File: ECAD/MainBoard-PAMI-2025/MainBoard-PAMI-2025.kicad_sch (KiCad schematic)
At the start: 52 parts, among them J10 Serial, J11 Con_Batt, J13 OLED, J2 USB_B, J3 Sensor_RIGHT, J4 Servo, J5 Sensor_LEFT, J6 Servo, J7 LeftMotor, J8 RightMotor, SW1 SW_SPDT, SW2 SW_Reed, SW3 SW_SPDT, SW4 SW_DIP_x02, U1 ESP32-S3-WROOM-1, U3 TMC2208_SILENTSTEPSTICK, U4 TMC2208_SILENTSTEPSTICK, U5 R-78E3.3-1.0

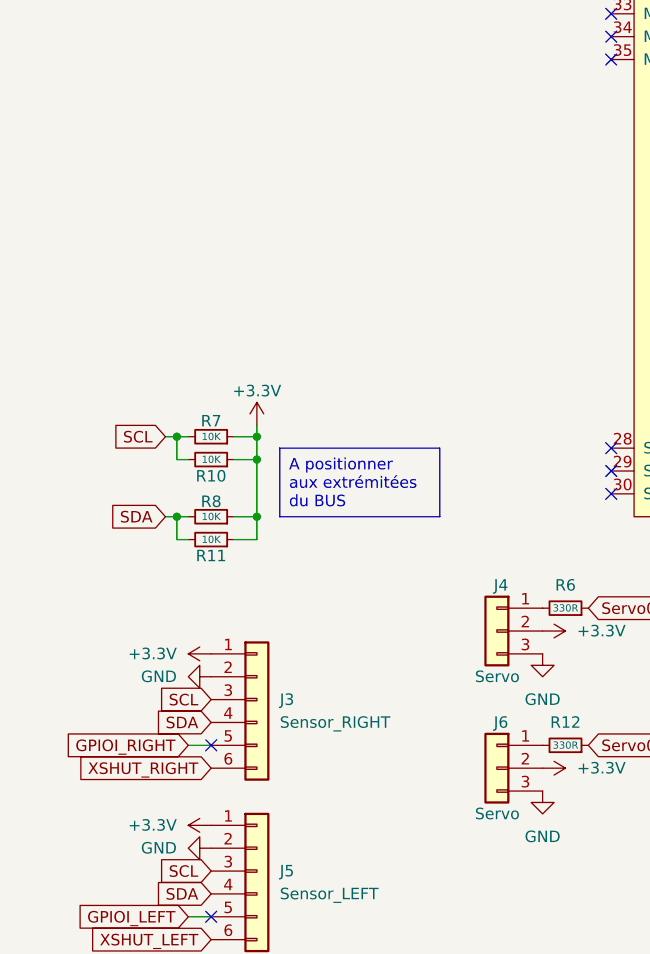
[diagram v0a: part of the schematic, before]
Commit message: add sensor center
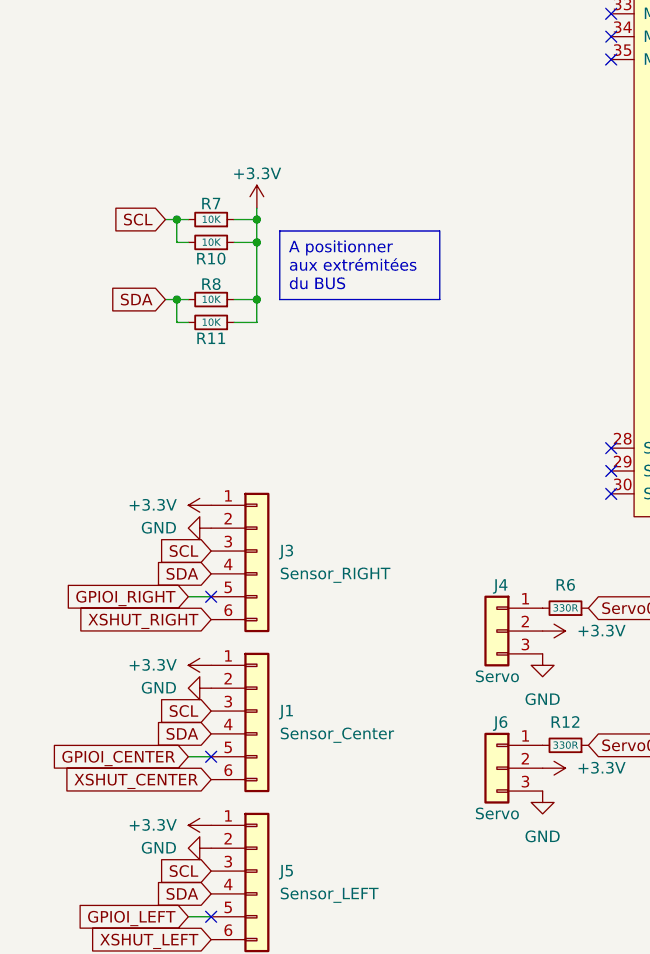
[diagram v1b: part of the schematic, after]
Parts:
- added J1: Sensor_Center, Connector_PinSocket_2.54mm:PinSocket_1x06_P2.54mm_Vertical, symbol Connector_Generic:Conn_01x06
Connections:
- net +3.3V: now also J1.1 (Pin_1)
- net GND: now also J1.2 (Pin_2)
- net SCL: now also J1.3 (Pin_3)
- net SDA: now also J1.4 (Pin_4)
- new net GPIOI_CENTER: J1.5 (Pin_5)
- new net XSHUT_CENTER: J1.6 (Pin_6)
- no-connect marks 19 -> 20
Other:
- moved on the sheet: J3, R10, R11, R7, R8
